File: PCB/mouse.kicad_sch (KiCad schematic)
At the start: 16 parts, among them SW1 SW_Push, U2 nice_nano

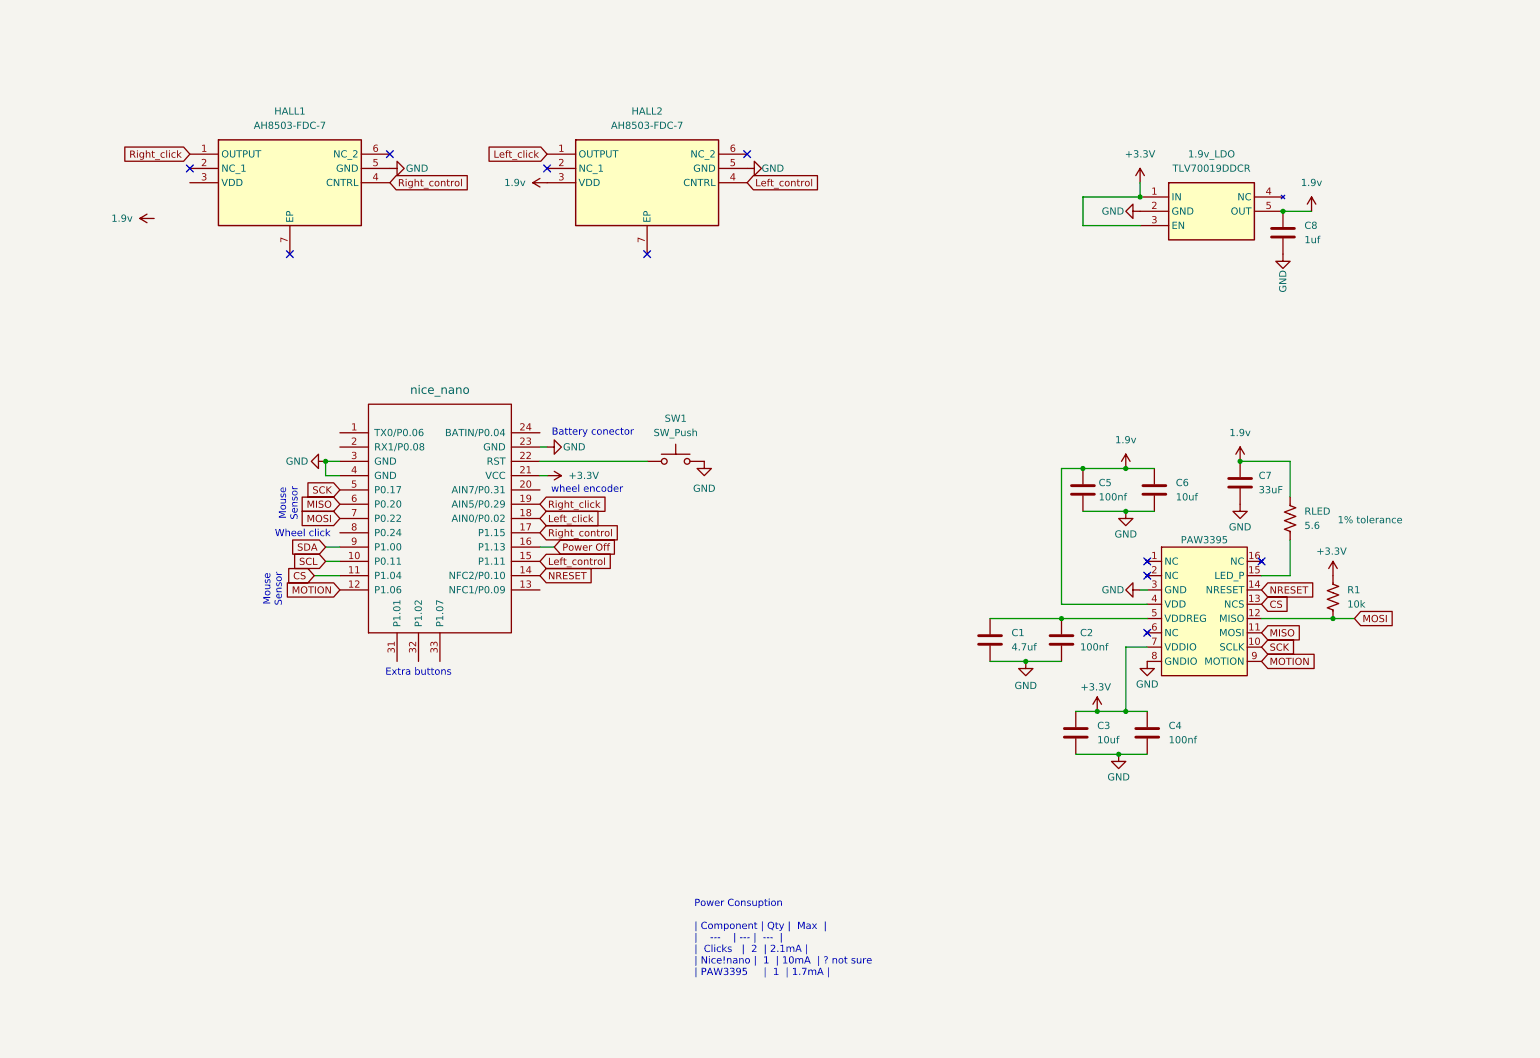
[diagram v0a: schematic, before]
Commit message: En proceso
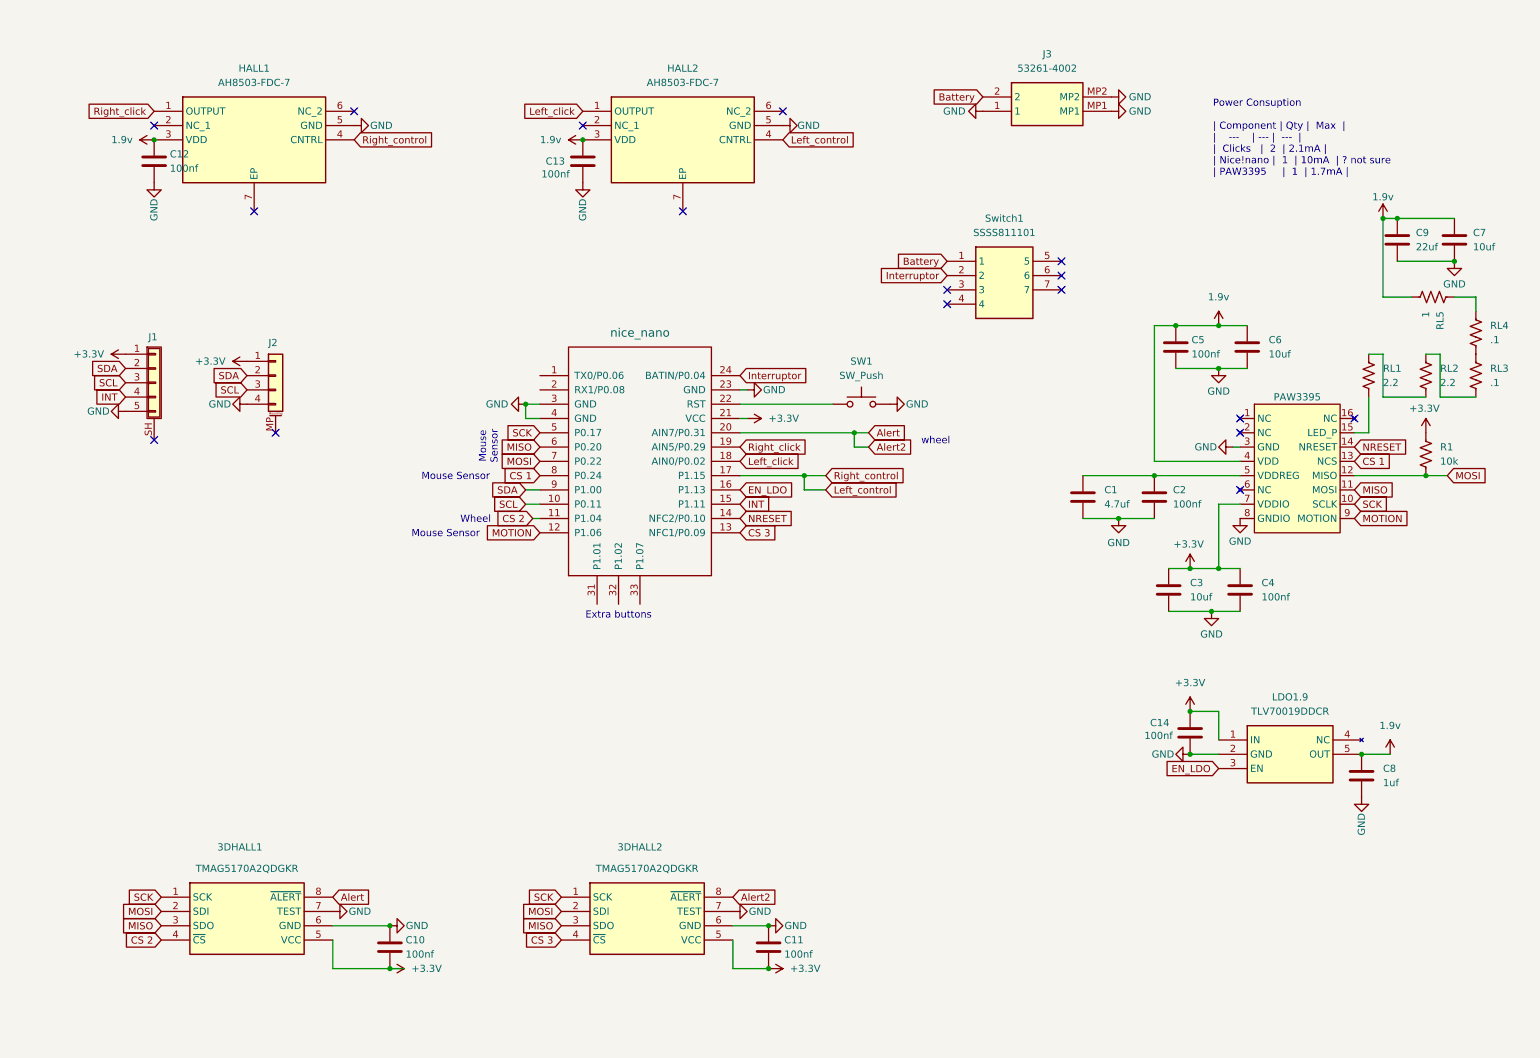
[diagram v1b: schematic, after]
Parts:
- added 3DHALL1, 3DHALL2: TMAG5170A2QDGKR, TMAG5170A2QDGKR:SOP65P490X110-8N, symbol TMAG5170A2QDGKR:TMAG5170A2QDGKR
- added C10, C11, C12, C13, C14: 100nf, Capacitor_SMD:C_0805_2012Metric, symbol Device:C
- added C9: 22uf, Capacitor_SMD:C_0805_2012Metric, symbol Device:C
- added J1: Conn_01x05_Shielded, Connector_PinHeader_2.54mm:PinHeader_1x05_P2.54mm_Vertical, symbol Connector_Generic_Shielded:Conn_01x05_Shielded
- added J2: Conn_01x04_MountingPin, Connector_JST:JST_SH_SM04B-SRSS-TB_1x04-1MP_P1.00mm_Horizontal, symbol Connector_Generic_MountingPin:Conn_01x04_MountingPin
- added J3: 53261-4002, 53261-4002:532614002, symbol 53261-4002:53261-4002
- added RL2: 2.2, Resistor_SMD:R_0805_2012Metric, symbol Device:R_US
- added RL3, RL4: .1, Resistor_SMD:R_0805_2012Metric, symbol Device:R_US
- added RL5: 1, Resistor_SMD:R_0805_2012Metric, symbol Device:R_US
- added Switch1: SSSS811101, SSSS811101:SSSS811101, symbol SSSS811101:SSSS811101
- C1, C2, C3, C4, C5, C6, C8: footprint (none) -> Capacitor_SMD:C_0805_2012Metric
- C7: value 33uF -> 10uf; footprint (none) -> Capacitor_SMD:C_0805_2012Metric
- LDO1.9: renamed from 1.9v_LDO; footprint SOT95P280X110-5N -> SOT95P280X110-5N:SOT95P280X110-5N
- R1: footprint (none) -> Resistor_SMD:R_0805_2012Metric
- RL1: renamed from RLED; value 5.6 -> 2.2; footprint (none) -> Resistor_SMD:R_0805_2012Metric
- SW1: footprint (none) -> PCM_JLCPCB:SW_TS-1088-AR02016
- U2: footprint KiCad:nice_nano -> Nice_nano:nice_nano
- renumbered OpticalSensor to OpticalSensor1
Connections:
- net Right_control is gone; now on net Left_control: HALL1.4 (CNTRL), U2.17 (P1.15)
- net +3.3V: now also 3DHALL1.5 (VCC), 3DHALL2.5 (VCC), C10.2, C11.2, C14.1, J1.1 (Pin_1), J2.1 (Pin_1); no longer LDO1.9.3 (EN)
- net 1.9v: now also HALL1.3 (VDD), C12.1, C13.1, C9.1, RL5.1; no longer RL1.2
- net GND: now also 3DHALL1.6 (GND), 3DHALL1.7 (TEST), 3DHALL2.6 (GND), 3DHALL2.7 (TEST), C10.1, C11.1, C12.2, C13.2, C14.2, C9.2, J1.5 (Pin_5), J2.4 (Pin_4), J3.1, J3.MP1, J3.MP2
- net Left_control: no longer U2.15 (P1.11)
- net MISO: now also 3DHALL1.3 (SDO), 3DHALL2.3 (SDO)
- net MOSI: now also 3DHALL1.2 (SDI), 3DHALL2.2 (SDI)
- net SCK: now also 3DHALL1.1 (SCK), 3DHALL2.1 (SCK)
- net SCL: now also J1.3 (Pin_3), J2.3 (Pin_3)
- net SDA: now also J1.2 (Pin_2), J2.2 (Pin_2)
- net CS 3: now reaches U2.13 (NFC1/P0.09)
- net CS 3: now also 3DHALL2.4 (~{CS})
- net Alert: now reaches U2.20 (AIN7/P0.31)
- net Alert: now also 3DHALL1.8 (~{ALERT}), 3DHALL2.8 (~{ALERT})
- net Interruptor: now reaches U2.24 (BATIN/P0.04)
- net Interruptor: now also Switch1.2
- net CS 1: now reaches U2.8 (P0.24)
- net CS 1: now also OpticalSensor1.13 (NCS)
- net CS renamed CS 2
- net CS 2: now also 3DHALL1.4 (~{CS}); no longer OpticalSensor1.13 (NCS)
- net Power Off renamed EN_LDO
- net EN_LDO: now also LDO1.9.3 (EN)
- new net: RL4.2, RL5.2
- new net: RL3.2, RL4.1
- new net: RL1.2, RL2.1
- new net: RL2.2, RL3.1
- new net Battery: J3.2, Switch1.1
- new net INT: J1.4 (Pin_4), U2.15 (P1.11)
- no-connect marks 10 -> 17
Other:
- note added: "Wheel"
- note added: "wheel"
- note removed: "Battery conector"
- note removed: "Wheel click"
- note removed: "wheel encoder"
- moved on the sheet: C1, C2, C3, C4, C5, C6, C7, C8, HALL1, HALL2, LDO1.9, R1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

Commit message: bk
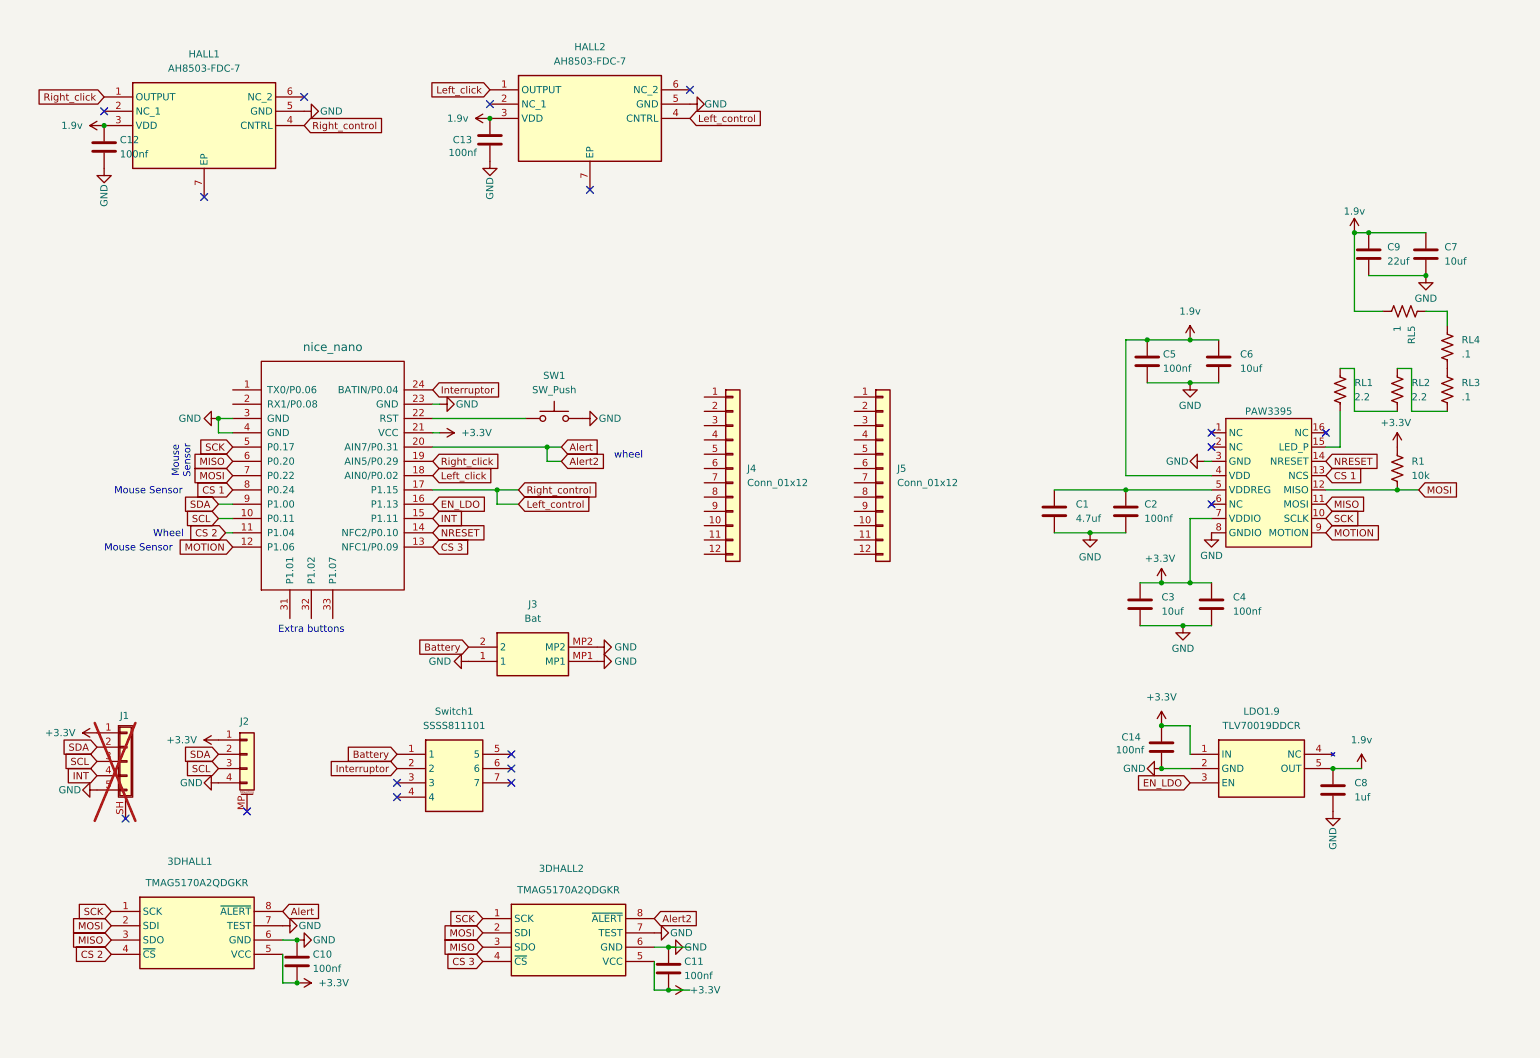
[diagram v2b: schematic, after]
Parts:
- added J4, J5: Conn_01x12, Connector_PinSocket_2.54mm:PinSocket_1x12_P2.54mm_Vertical, symbol Connector_Generic:Conn_01x12
- 3DHALL1: JLC-PCB (none) -> C3716101; Jst https://jlcpcb.com/partdetail/TexasInstruments-TMAG5170A2QD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 -> (none); Mouser Part Number 595-TMAG5170A2QDGKR -> (none); Mouser Price/Stock https://www.mouser.co.uk/ProductDetail/Texas-Instruments/TM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 -> (none)
- 3DHALL2: JLC-PCB (none) -> C3716101; Mouser Part Number 595-TMAG5170A2QDGKR -> (none); Mouser Price/Stock https://www.mouser.co.uk/ProductDetail/Texas-Instruments/TM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 -> (none)
- C1: JLC-PCB (none) -> C1779
- C10, C11, C12, C13, C14, C2, C4, C5: JLC-PCB (none) -> C28233
- C3, C6, C7: JLC-PCB (none) -> C15850
- C8: JLC-PCB (none) -> C28323
- C9: JLC-PCB (none) -> C45783
- HALL1, HALL2: JLC-PCB C842153 -> C842150; Mouser Part Number 621-AH8503-FDC-7 -> (none); Mouser Price/Stock https://www.mouser.co.uk/ProductDetail/Diodes-Incorporated/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 -> (none)
- J1: now not fitted; now left out of the parts list
- J2: JLC-PCB (none) -> C160404
- J3: value 53261-4002 -> Bat; JLC-PCB (none) -> C17559503; Mouser Part Number 538-53261-4002 -> (none); Mouser Price/Stock https://www.mouser.co.uk/ProductDetail/Molex/53261-4002?qs=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 -> (none)
- LDO1.9: JLC-PCB (none) -> C2862411; Mouser Part Number 595-TLV70019DDCR -> (none); Mouser Price/Stock https://www.mouser.co.uk/ProductDetail/Texas-Instruments/TL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 -> (none)
- OpticalSensor1: footprint lib:DIP-16_PAW3395 -> PAW3395:DIP-16_PAW3395; JLC-PCB (none) -> C41346211
- R1: JLC-PCB (none) -> C17414
- RL1, RL2: JLC-PCB (none) -> C17521
- RL3, RL4: footprint Resistor_SMD:R_0805_2012Metric -> Resistor_SMD:R_1206_3216Metric; JLC-PCB (none) -> C25334
- RL5: JLC-PCB (none) -> C25271
- SW1: JLC-PCB (none) -> C720477
- Switch1: JLC-PCB (none) -> C97433; Mouser Part Number 688-SSSS811101 -> (none); Mouser Price/Stock https://www.mouser.co.uk/ProductDetail/Alps-Alpine/SSSS8111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 -> (none)
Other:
- note removed: "Power Consuption | Component | Qty | Max | | --- | --- | --- | | Clicks | 2 | 2.1mA | | Nice!nano | 1 | 10mA | ? not sure | PAW3395 | 1 | 1.7mA |"
- moved on the sheet: 3DHALL1, 3DHALL2, C1, C10, C11, C12, C13, C14, C2, C3, C4, C5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

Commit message: bk
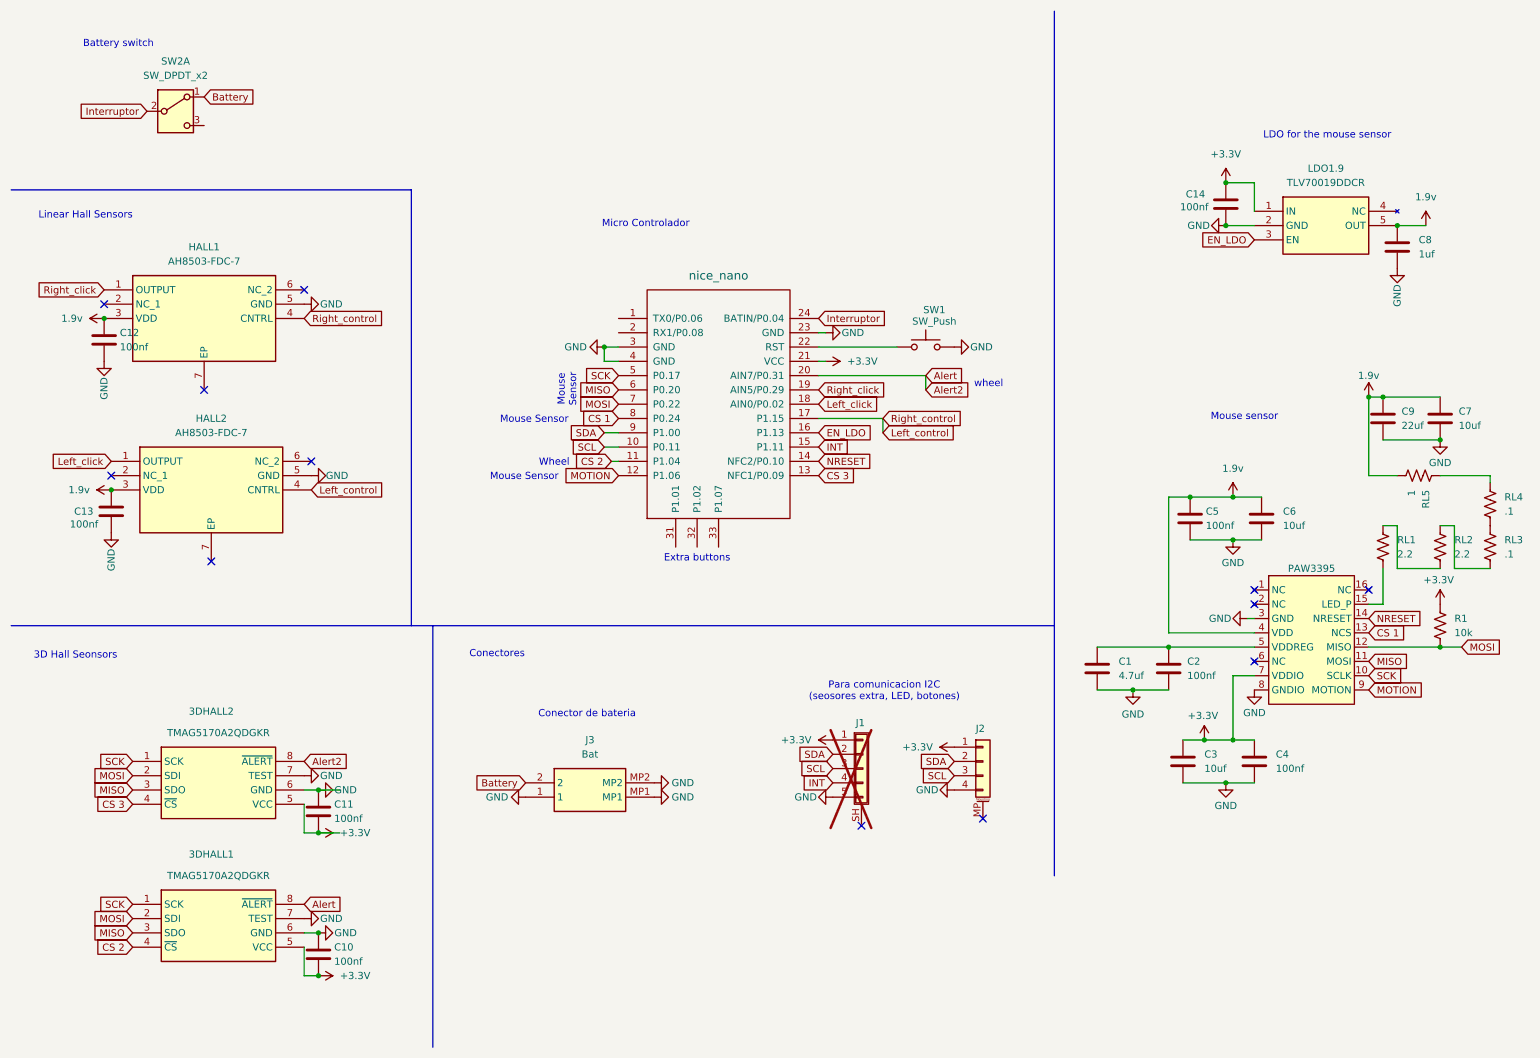
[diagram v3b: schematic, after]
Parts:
- removed J4, J5: Conn_01x12, Connector_PinSocket_2.54mm:PinSocket_1x12_P2.54mm_Vertical, symbol Connector_Generic:Conn_01x12
- removed Switch1: SSSS811101, SSSS811101:SSSS811101, symbol SSSS811101:SSSS811101
- added SW2: SW_DPDT_x2, SSSS811101:SSSS811101, symbol Switch:SW_DPDT_x2
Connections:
- net Battery: now also SW2.1 (A)
- net Interruptor: now also SW2.2 (B)
- no-connect marks 17 -> 12
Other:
- note added: "3D Hall Seonsors"
- note added: "Battery switch"
- note added: "Conector de bateria"
- note added: "Conectores"
- note added: "LDO for the mouse sensor"
- note added: "Linear Hall Sensors"
- note added: "Micro Controlador"
- note added: "Mouse sensor"
- note added: "Para comunicacion I2C (seosores extra, LED, botones)"
- moved on the sheet: 3DHALL1, 3DHALL2, C1, C10, C11, C12, C13, C14, C2, C3, C4, C5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
